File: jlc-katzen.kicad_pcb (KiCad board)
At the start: 2 copper layers, 55 x 45 mm, 62 parts, among them J1 USB_C_Receptacle_USB2.0_16P, J2 Conn_01x04, J3 Conn_01x04, J4 Conn_01x02, J5 Conn_ARM_SWD_TagConnect_TC2030, Q1 2N7002, Q2 2N7002, Q3 2N7002, U1 XC6206P332MR, U2 W25Q128JVSIQ, U3 RP2040, U4 IRM-H638T/TR2, Y1 12 MHz 20 pF X322512MSB4SI

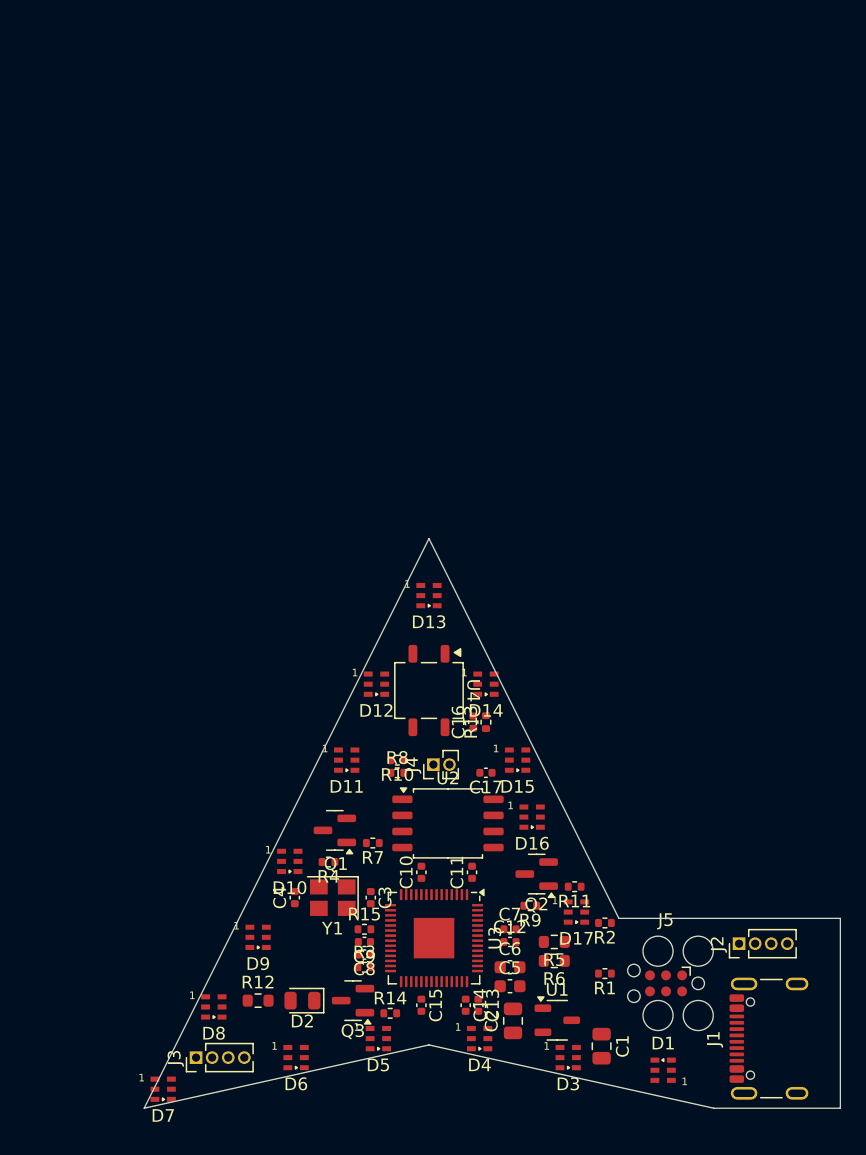
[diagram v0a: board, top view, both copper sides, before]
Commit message: rough route
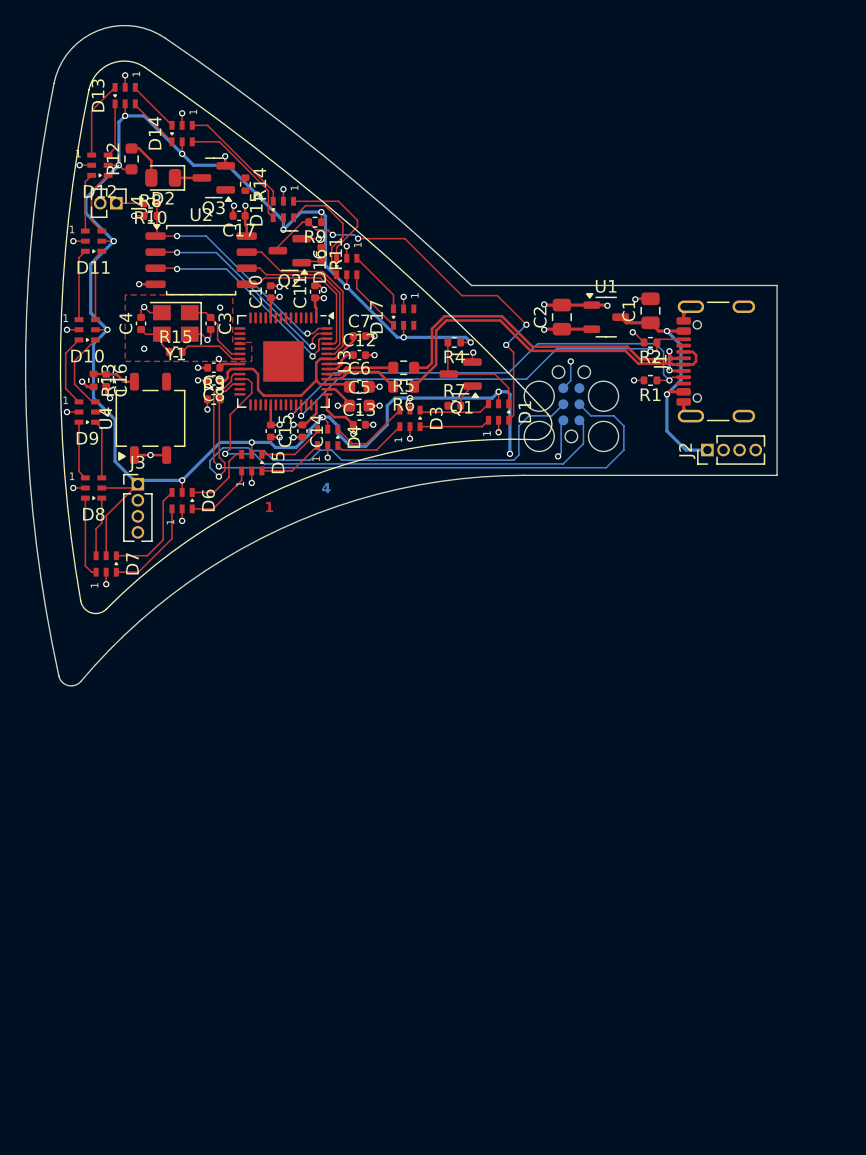
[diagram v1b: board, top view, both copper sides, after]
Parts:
- J5: moved to B.Cu
- moved R12 67.2 mm to (99.0, 75.0), turned to 90 degrees
- moved R14 66.5 mm to (108.0, 77.0), turned to -90 degrees
- moved D2 65.9 mm to (101.5, 76.5)
- moved Q3 65.9 mm to (105.5, 76.5)
- moved C1 58.2 mm to (140.0, 87.0), turned to 90 degrees
- moved R9 56.6 mm to (113.5, 80.0)
- moved C2 55.7 mm to (133.0, 87.5)
- moved U1 55.7 mm to (136.5, 87.5)
- moved R11 53.9 mm to (114.0, 82.5), turned to -90 degrees
- moved J1 53.7 mm to (146.3, 91.0)
- moved D1 53.6 mm to (128.0, 95.0), turned to 90 degrees
- moved Q2 53.0 mm to (111.5, 82.2)
- moved D3 52.0 mm to (121.0, 95.5), turned to 90 degrees
- moved J4 50.9 mm to (97.8, 78.5), turned to -90 degrees
- moved D14 49.7 mm to (103.0, 73.0), turned to -90 degrees
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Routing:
- net +5V: track 0.00 -> 176.3 mm, vias 0 -> 19
- net GND: track 0.00 -> 50.4 mm, vias 0 -> 44
- net /SWCLK: track 0.00 -> 47.6 mm, vias 0 -> 1
- net /~{RESET}: track 0.00 -> 42.9 mm, vias 0 -> 1
- net /SWDIO: track 0.00 -> 38.8 mm, vias 0 -> 1
- net /CC1: track 0.00 -> 37.8 mm, vias 0 -> 2
- net +3.3V: track 0.00 -> 35.9 mm, vias 0 -> 13
- net /CC2: track 0.00 -> 34.1 mm, vias 0 -> 2
- net /LED_DAT_5V: track 0.00 -> 32.7 mm, vias 0 -> 4
- net /USB_D+: track 0.00 -> 30.2 mm, vias 0 -> 2
- net /USB_D-: track 0.00 -> 29.1 mm
- net /FLASH_~{SS}: track 0.00 -> 19.5 mm, vias 0 -> 2
- net +1V1: track 0.00 -> 18.6 mm
- net /FLASH_D2: track 0.00 -> 17.5 mm, vias 0 -> 2
- net /FLASH_D1: track 0.00 -> 17.4 mm, vias 0 -> 2
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- added copper zone on In2.Cu, net +3.3V
- added copper zone on F.Cu, net GND
- added copper zone on In1.Cu, net GND
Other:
- board size 55 x 45 mm -> 59.4 x 52.2 mm
- copper layers 2 -> 4
- board text added: "1"
- board text added: "2"
- board text added: "3"
- board text added: "4"
- board text added: "Chuuni Rights!"
